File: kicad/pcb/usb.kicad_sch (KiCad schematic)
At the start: 38 parts, among them J2 USB Connector, U1 FE1.1, U5 MIC2026-2BM, U6 USBLC6-2P6, Y1 12 MHz

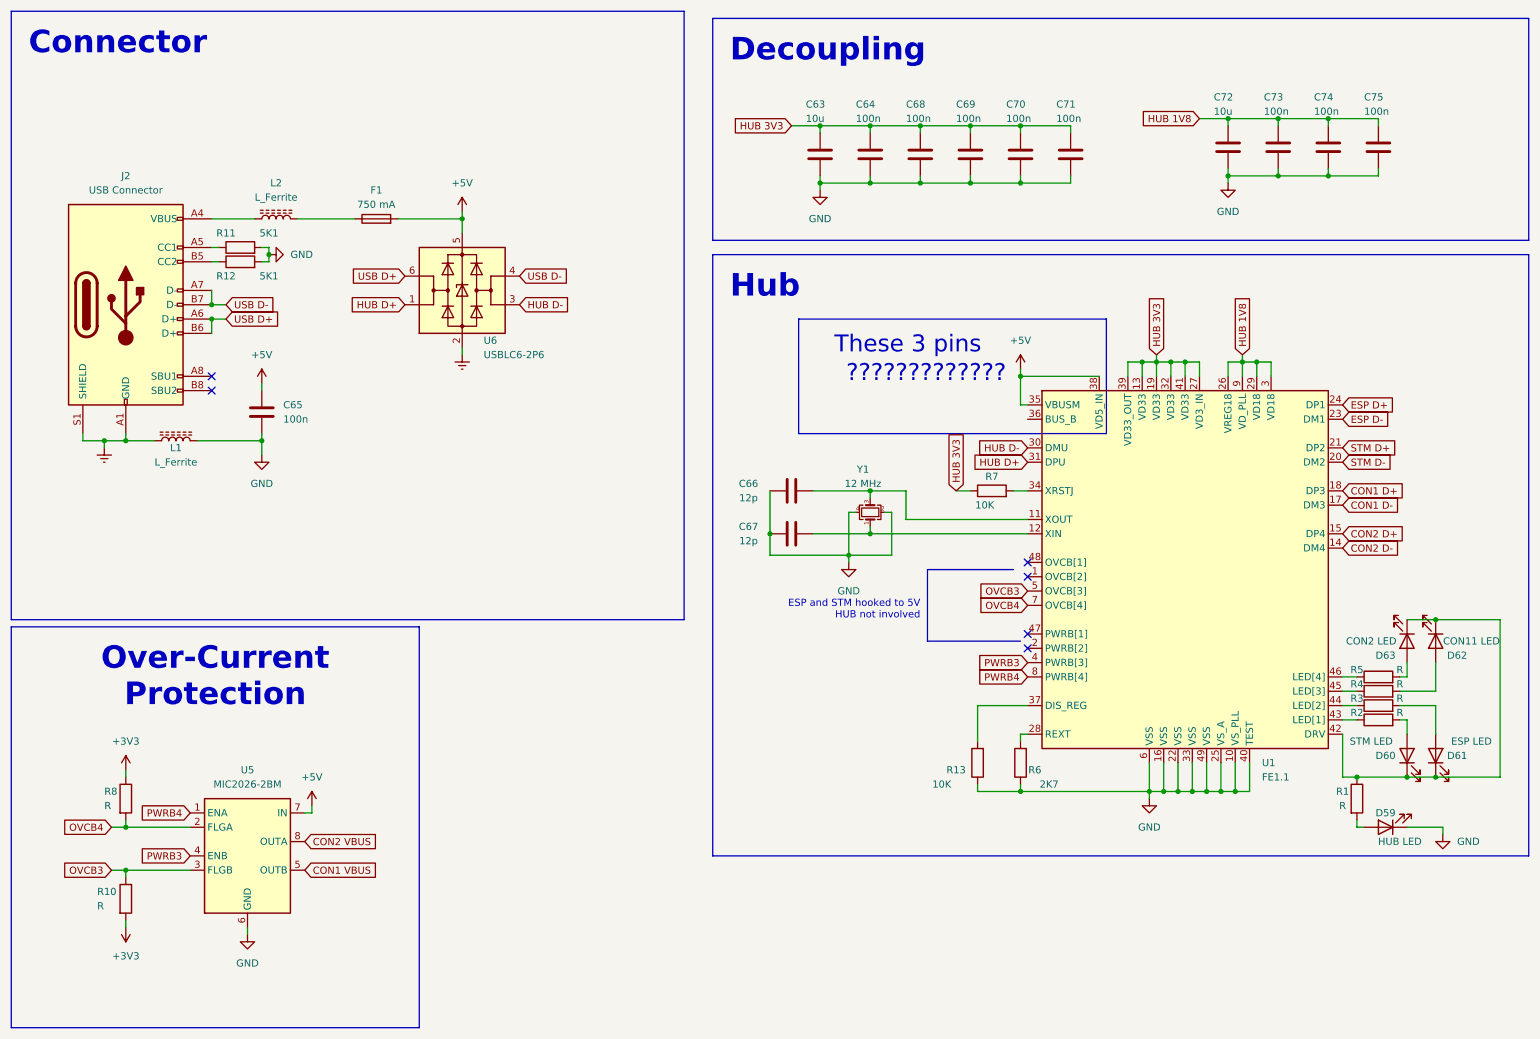
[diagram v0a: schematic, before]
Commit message: (WIP) Tracing v2
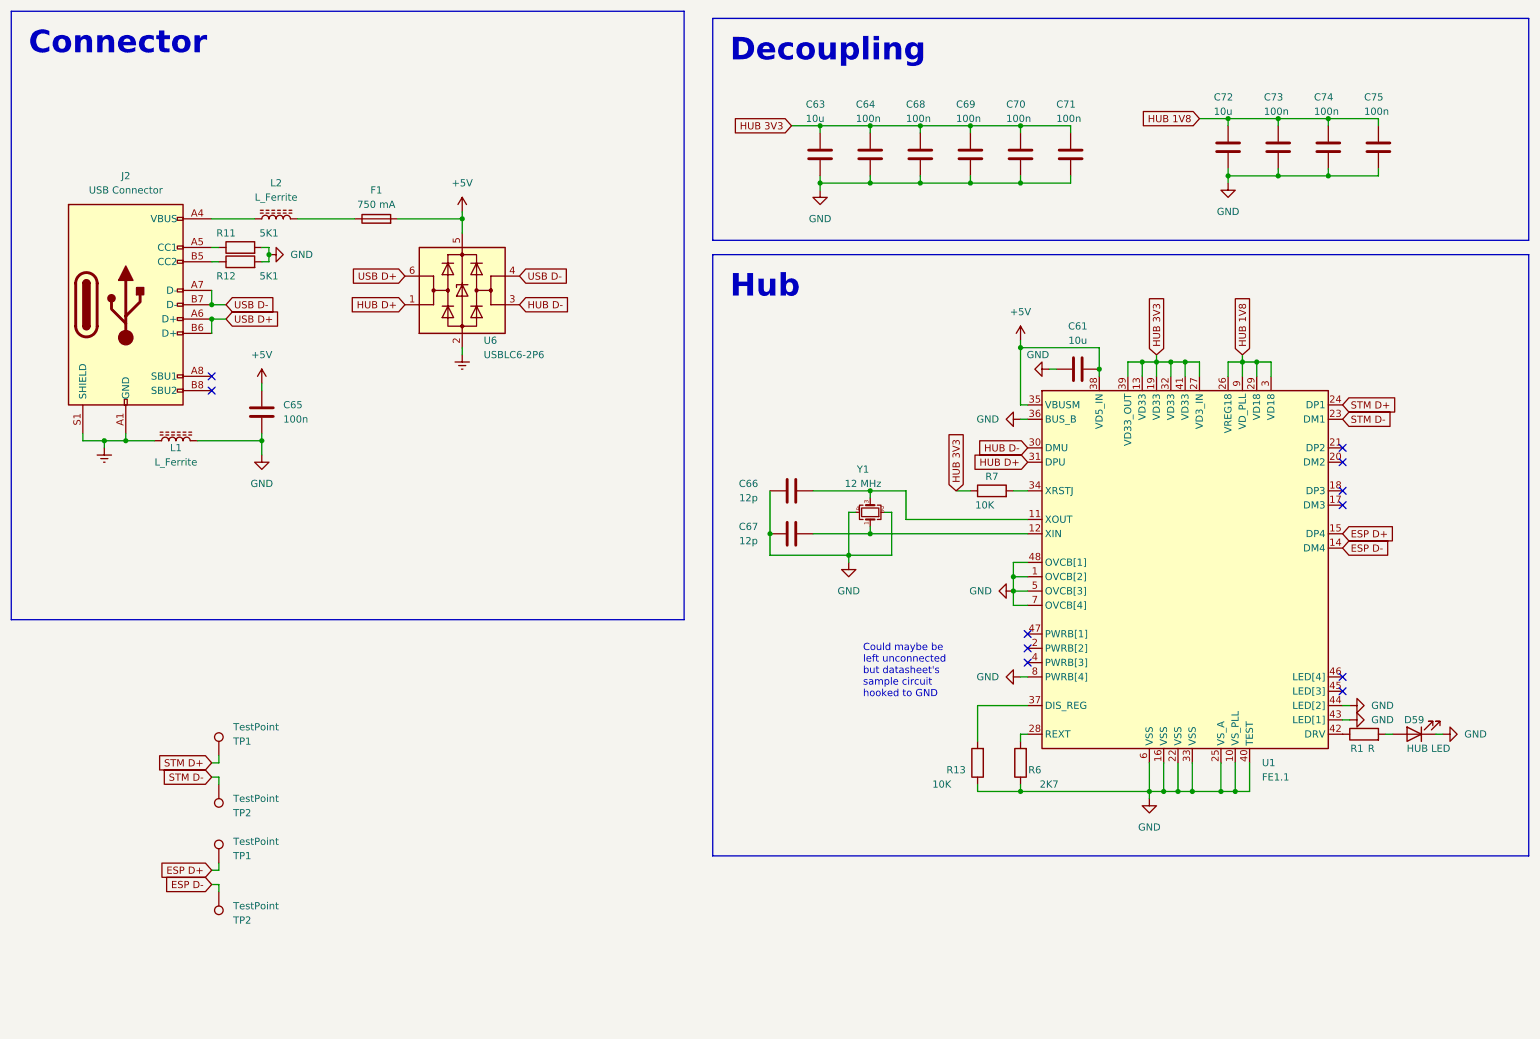
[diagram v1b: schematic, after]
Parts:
- removed D60: STM LED, symbol Device:LED
- removed D61: ESP LED, symbol Device:LED
- removed D62: CON11 LED, symbol Device:LED
- removed D63: CON2 LED, symbol Device:LED
- removed R10, R2, R3, R4, R5, R8: R, Resistor_SMD:R_0402_1005Metric_Pad0.72x0.64mm_HandSolder, symbol Device:R
- removed U5: MIC2026-2BM, Package_DIP:DIP-8_W7.62mm, symbol Power_Management:MIC2026-2BM
- added C61: 10u, Capacitor_SMD:C_0402_1005Metric_Pad0.74x0.62mm_HandSolder, symbol Device:C
- added TP1 (x2), TP2 (x2): TestPoint, TestPoint:TestPoint_Pad_D2.0mm, symbol Connector:TestPoint
- D59: footprint (none) -> LED_SMD:LED_0402_1005Metric_Pad0.77x0.64mm_HandSolder
- F1: footprint (none) -> Fuse:Fuse_0402_1005Metric_Pad0.77x0.64mm_HandSolder
- L1, L2: footprint (none) -> Inductor_SMD:L_0402_1005Metric_Pad0.77x0.64mm_HandSolder
- Y1: footprint Crystal:Crystal_SMD_2016-4Pin_2.0x1.6mm -> Crystal:Crystal_SMD_3225-4Pin_3.2x2.5mm
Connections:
- net CON2 D+ is gone; now on net ESP D+: U1.15 (DP4)
- net CON2 D- is gone; now on net ESP D-: U1.14 (DM4)
- net OVCB3 is gone; now on net GND: U1.5 (OVCB[3])
- net OVCB4 is gone; now on net GND: U1.7 (OVCB[4])
- net PWRB4 is gone; now on net GND: U1.8 (PWRB[4])
- net +5V: now also C61.2
- net ESP D+: now also TP1.1; no longer U1.24 (DP1)
- net ESP D-: now also TP2.1; no longer U1.23 (DM1)
- net GND: now also U1.1 (OVCB[2]), U1.36 (BUS_B), U1.43 (LED[1]), U1.44 (LED[2]), U1.48 (OVCB[1]), C61.1; no longer U1.49 (VSS)
- net STM D+: now also U1.24 (DP1), TP1.1; no longer U1.21 (DP2)
- net STM D-: now also U1.23 (DM1), TP2.1; no longer U1.20 (DM2)
- net CON1 D+: no longer names the net of U1.18 (DP3)
- net CON1 D-: no longer names the net of U1.17 (DM3)
- net PWRB3: no longer names the net of U1.4 (PWRB[3])
- no-connect marks 6 -> 11
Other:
- note added: "Could maybe be left unconnected but datasheet's sample circuit hooked to GND"
- note removed: "?????????????"
- note removed: "ESP and STM hooked to 5V HUB not involved"
- note removed: "These 3 pins"
- moved on the sheet: D59, R1
